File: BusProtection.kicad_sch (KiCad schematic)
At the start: 84 parts, among them Q1 NX3008NBKS, Q10 MBT2222ADW1T1, Q11 NX3008NBKS, Q12 MBT2222ADW1T1, Q13 NX3008NBKS, Q14 MBT2222ADW1T1, Q15 NX3008NBKS, Q16 MBT2222ADW1T1, Q17 MMBT2907, Q18 MMBT2907, Q2 MBT2222ADW1T1, Q3 NX3008NBKS, Q4 MBT2222ADW1T1, Q5 NX3008NBKS, Q6 MBT2222ADW1T1, Q7 NX3008NBKS, Q8 MBT2222ADW1T1, Q9 NX3008NBKS

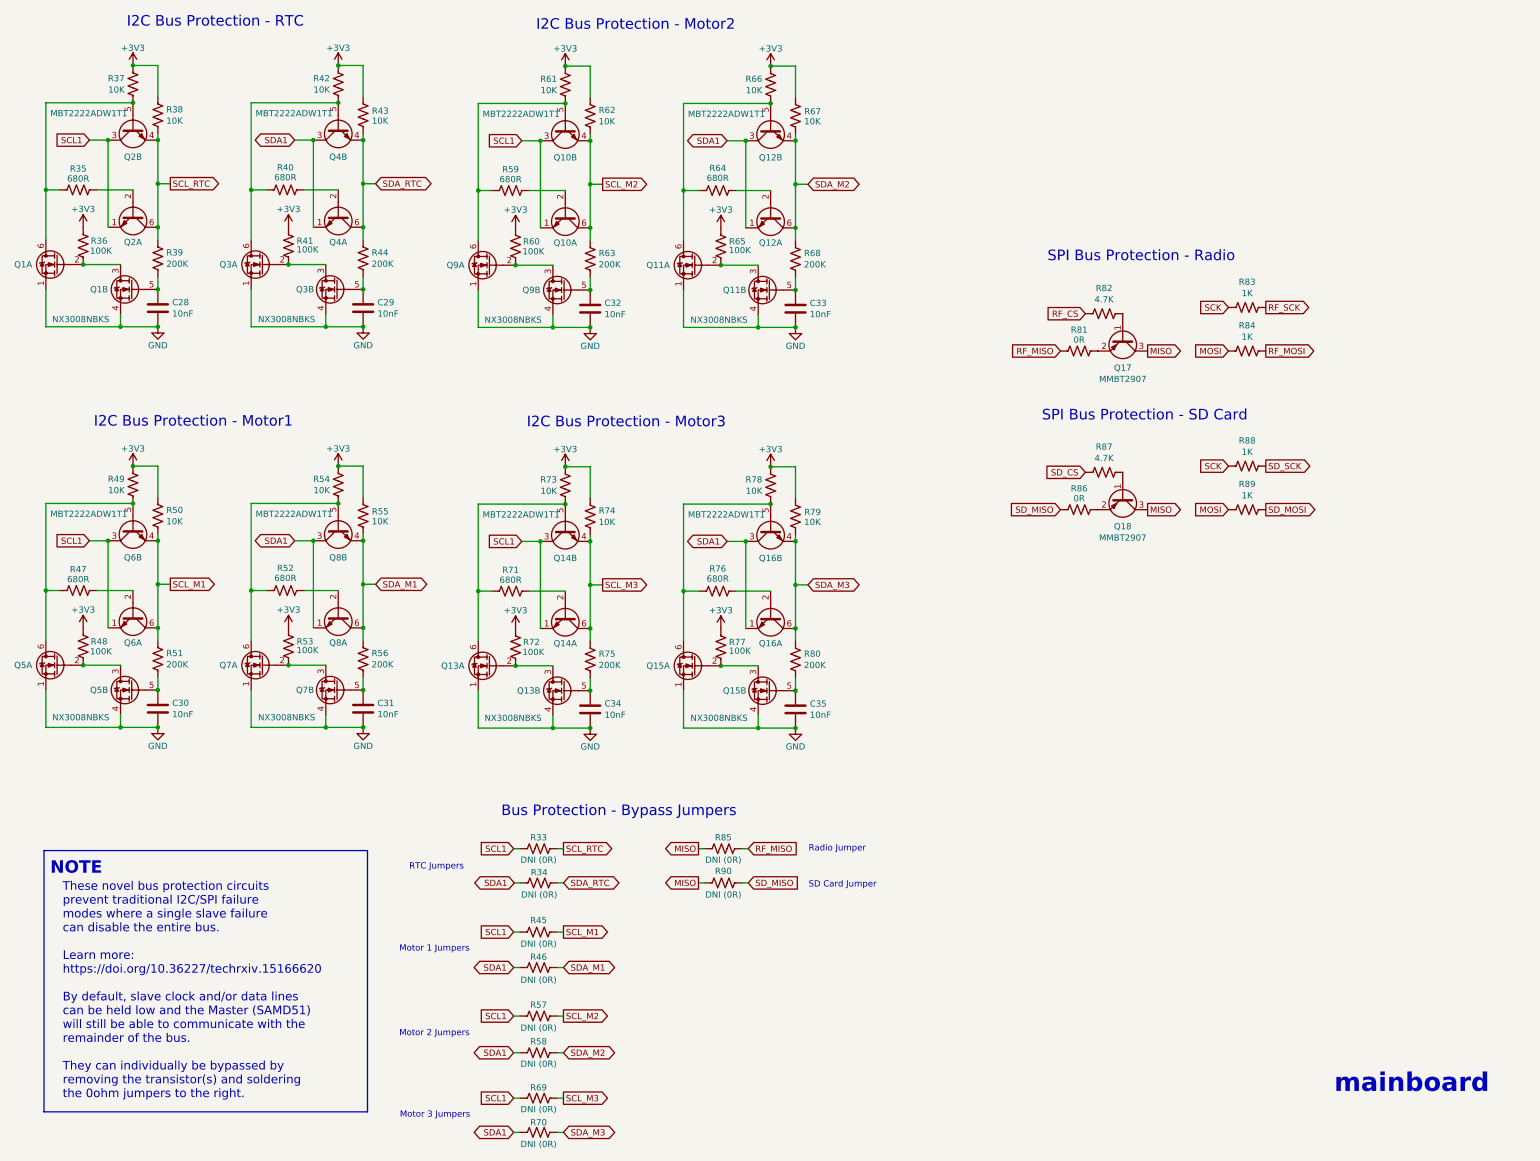
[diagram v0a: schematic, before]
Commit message: Stash C1 Updates
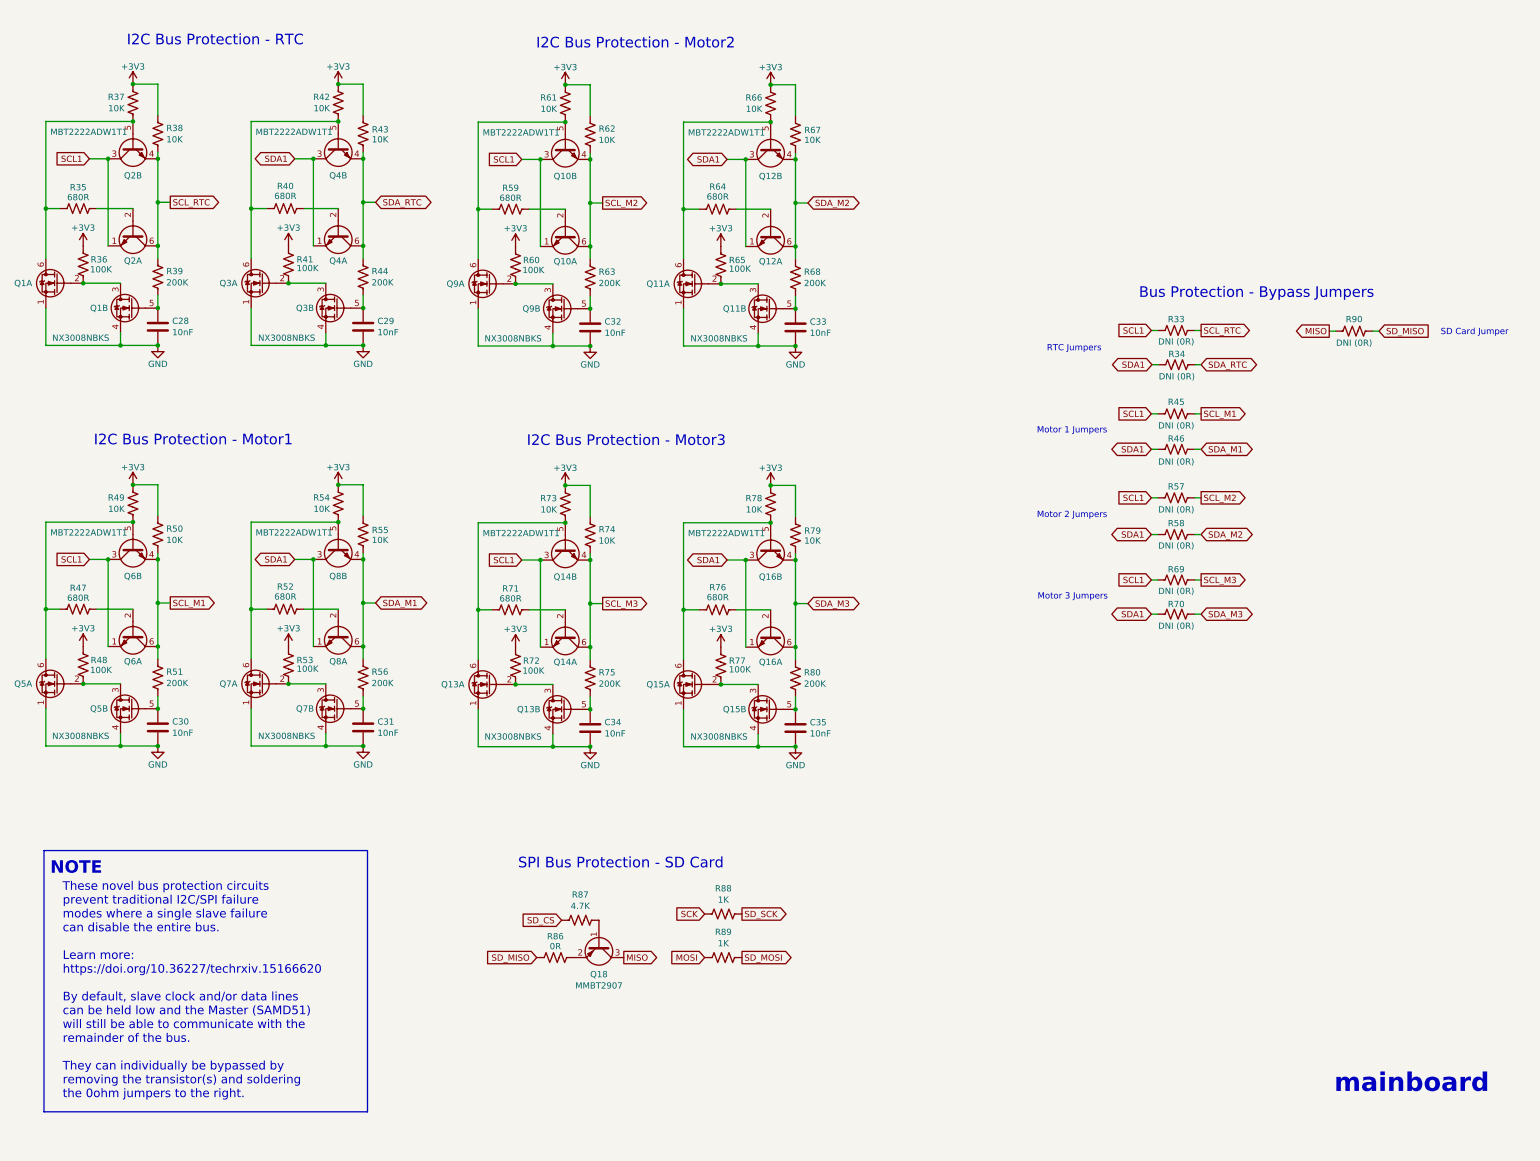
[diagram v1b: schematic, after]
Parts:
- removed Q17: MMBT2907, Package_TO_SOT_SMD:SOT-23, symbol mainboard:MMBT2907
- removed R81: 0R, Resistor_SMD:R_0603_1608Metric, symbol Device:R_US
- removed R82: 4.7K, Resistor_SMD:R_0603_1608Metric, symbol Device:R_US
- removed R83, R84: 1K, Resistor_SMD:R_0603_1608Metric, symbol Device:R_US
- removed R85: DNI (0R), Resistor_SMD:R_0603_1608Metric, symbol Device:R_US
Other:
- note removed: "Radio Jumper"
- note removed: "SPI Bus Protection - Radio"
- moved on the sheet: C28, C29, C30, C31, C32, C33, C34, C35, Q10A, Q10B, Q11A, Q11B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
